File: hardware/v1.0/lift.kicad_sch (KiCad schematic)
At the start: 13 parts, among them J8 Molex Mini Fit Jr 39-30-1060, U5 DRV8874PWPR

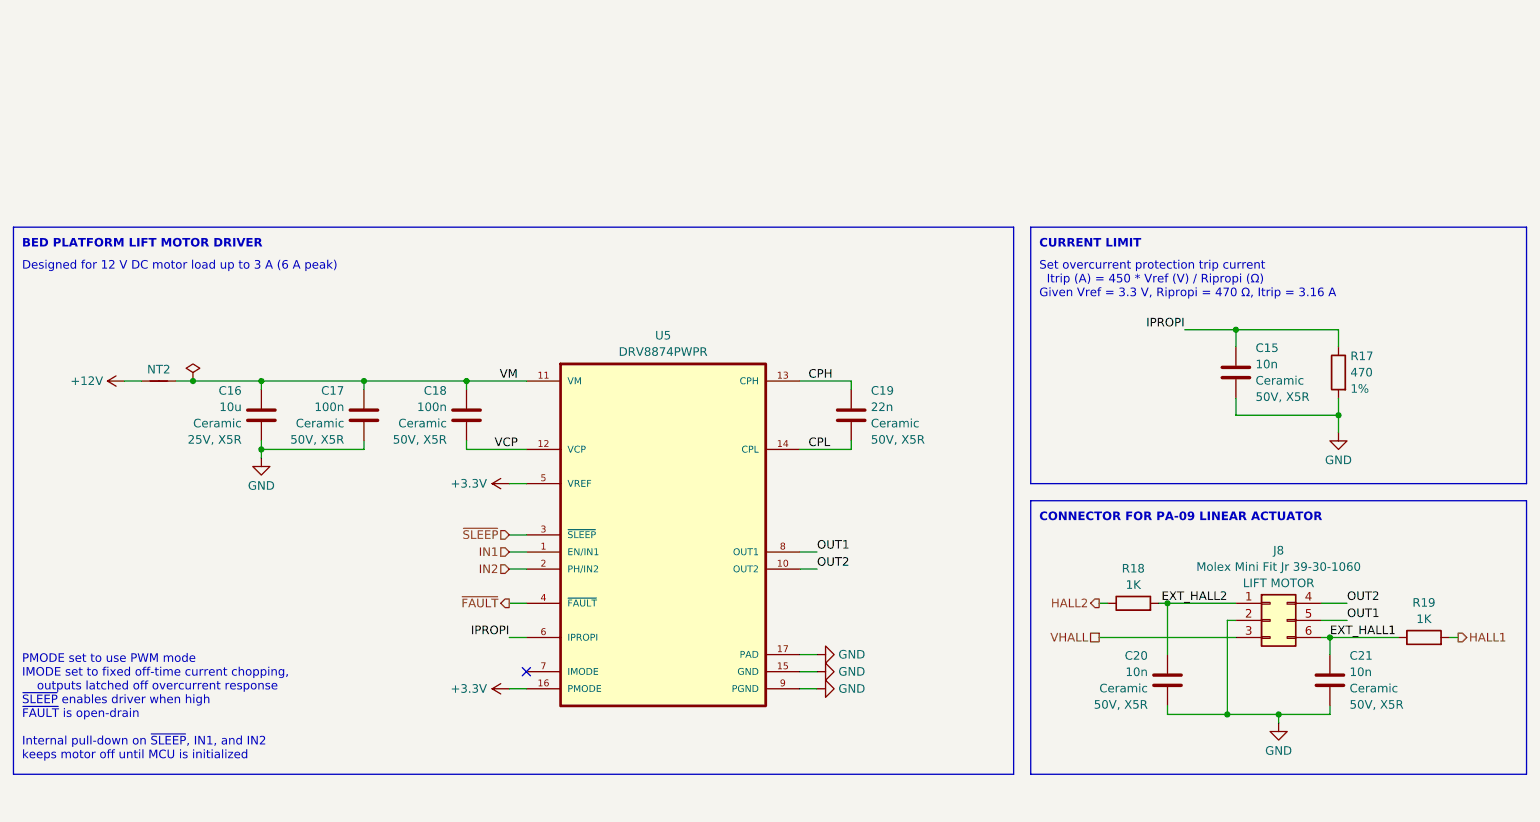
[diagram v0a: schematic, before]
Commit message: Complete first draft of v1.0 hardware.
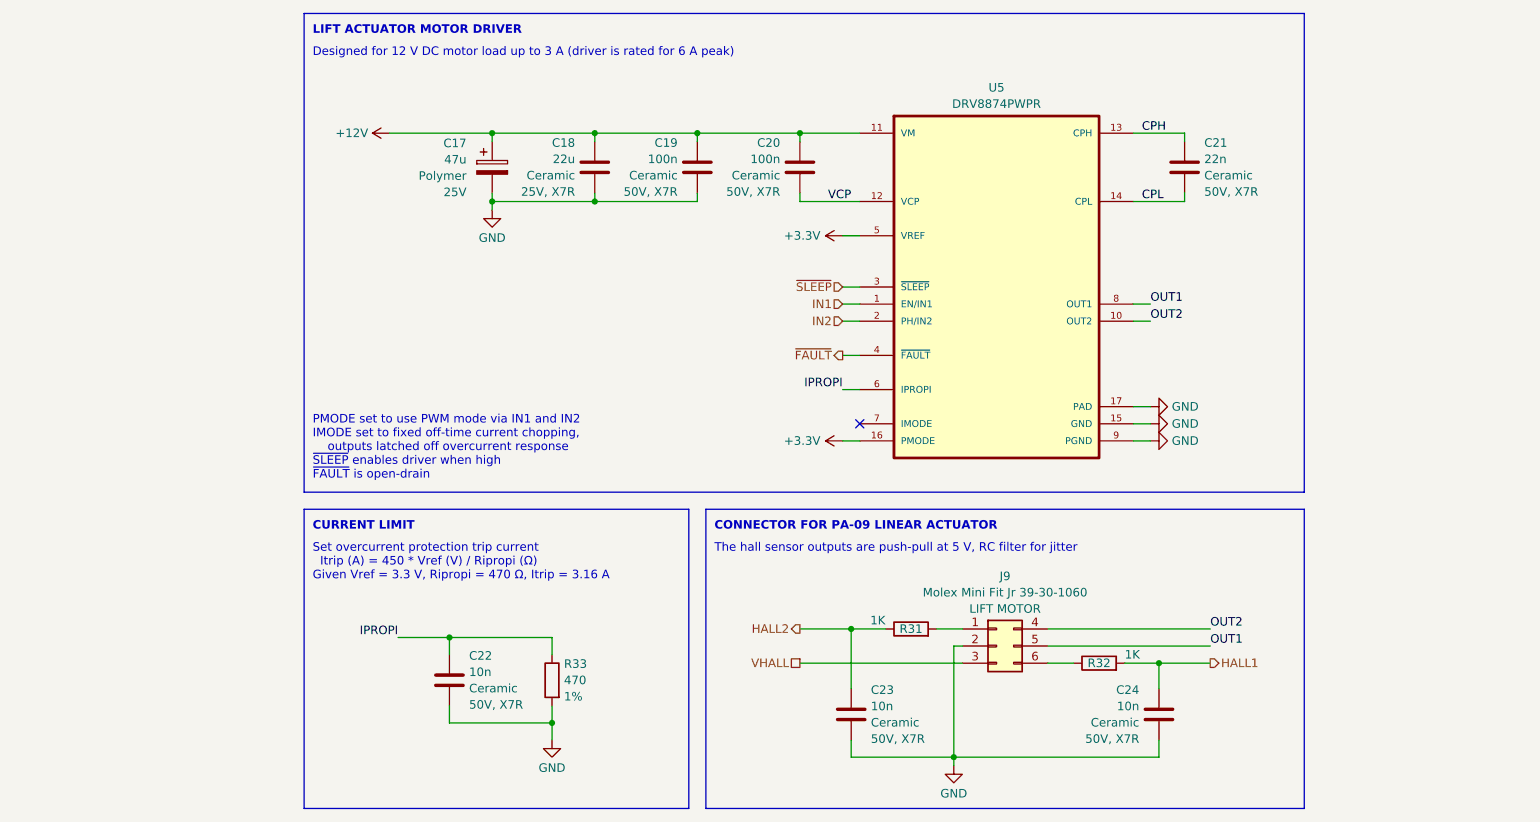
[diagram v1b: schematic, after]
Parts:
- removed C16: 10u, Capacitor_SMD:C_0805_2012Metric, symbol Device:C
- removed C20, C21: 10n, Capacitor_SMD:C_0603_1608Metric, symbol Device:C
- removed NT2: NetTie_2, Generic:NetTie-2_SMD_Pad2.5mm, symbol Device:NetTie_2
- added C17: 47u, Capacitor_THT:CP_Radial_D5.0mm_P2.50mm, symbol Device:C_Polarized
- added C18: 22u, Capacitor_SMD:C_1210_3225Metric, symbol Device:C
- added C23, C24: 10n, Capacitor_SMD:C_0603_1608Metric, symbol Device:C
- C19: renamed from C17; Rating 50V, X5R -> 50V, X7R
- C20: renamed from C18; Rating 50V, X5R -> 50V, X7R
- C21: renamed from C19; Rating 50V, X5R -> 50V, X7R
- C22: renamed from C15; Rating 50V, X5R -> 50V, X7R
- renumbered J8 to J9, R18 to R31, R19 to R32, R17 to R33
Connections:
- net VM is gone; now on net +12V: C19.1, C20.1, U5.11 (VM)
- net +12V: now also C17.1, C18.2
- net GND: now also C17.2, C18.1, C23.2, C24.2
- net HALL1: now also C24.1
- net HALL2: now also C23.1
- net EXT_HALL1: no longer names the net of J9.6 (Pin_6), R32.1
- net EXT_HALL2: no longer names the net of J9.1 (Pin_1), R31.2
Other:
- note added: "Designed for 12 V DC motor load up to 3 A (driver is rated for 6 A peak)"
- note added: "LIFT ACTUATOR MOTOR DRIVER"
- note added: "PMODE set to use PWM mode via IN1 and IN2 IMODE set to fixed off-time current chopping, outputs latched off overcurrent response ~{SLEEP} enables driver when high ~{FAULT} is open-drain"
- note added: "The hall sensor outputs are push-pull at 5 V, RC filter for jitter"
- note removed: "BED PLATFORM LIFT MOTOR DRIVER"
- note removed: "Designed for 12 V DC motor load up to 3 A (6 A peak)"
- note removed: "PMODE set to use PWM mode IMODE set to fixed off-time current chopping, outputs latched off overcurrent response ~{SLEEP} enables driver when high ~{FAULT} is open-drain Internal pull-down on ~{SLEEP}, IN1, and IN2 keeps motor off until MCU is initialized"
- moved on the sheet: C19, C20, C21, C22, J9, R31, R32, R33, U5
